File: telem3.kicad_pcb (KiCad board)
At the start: 4 copper layers, 124 x 80 mm, 200 parts, among them J1 STM32_TRACE, J10 Conn_01x04_Socket, J11 CAN_TERMINATION, J12 GPS_ANT, J3 EXPANSION_1, J4 ESP32_JTAG, J5 BAT, J6 STM_USBC, J7 Micro_SD_Card, J8 QT1, J9 QT2, Q1 2N7002, Q2 2N7002, Q3 2N7002, Q4 2N7002, Q5 2N7002, Q6 2N7002, Q7 IRLML9301, Q8 2N7002, SW1 RESET, SW2 OPT, SW3 ESP32_RST, SW4 GPS_RST, U1 STM32L562ZETx, U10 TCAN334G, U11 L80-R, U12 LSM6DS3, U13 BME280, U2 W25Q128JVS, U3 W25Q128JVS, U4 ESP32-C3-MINI-1, U5 TPS2116, U6 TPS54202DDC, U7 BQ24075RGT, U8 AP7361C-33E, U9 NUP4202, Y1 8MHz, Y2 32.768kHz

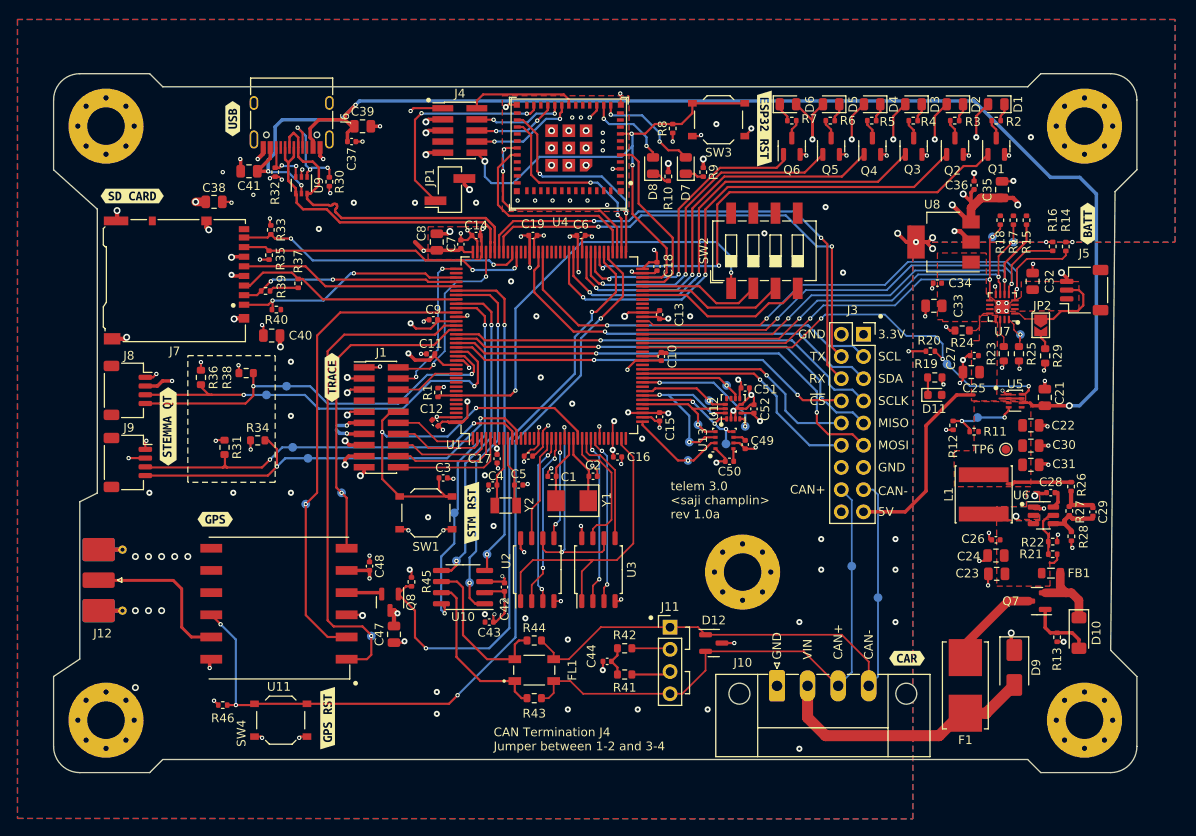
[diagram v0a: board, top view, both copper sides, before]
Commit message: fix uart gps
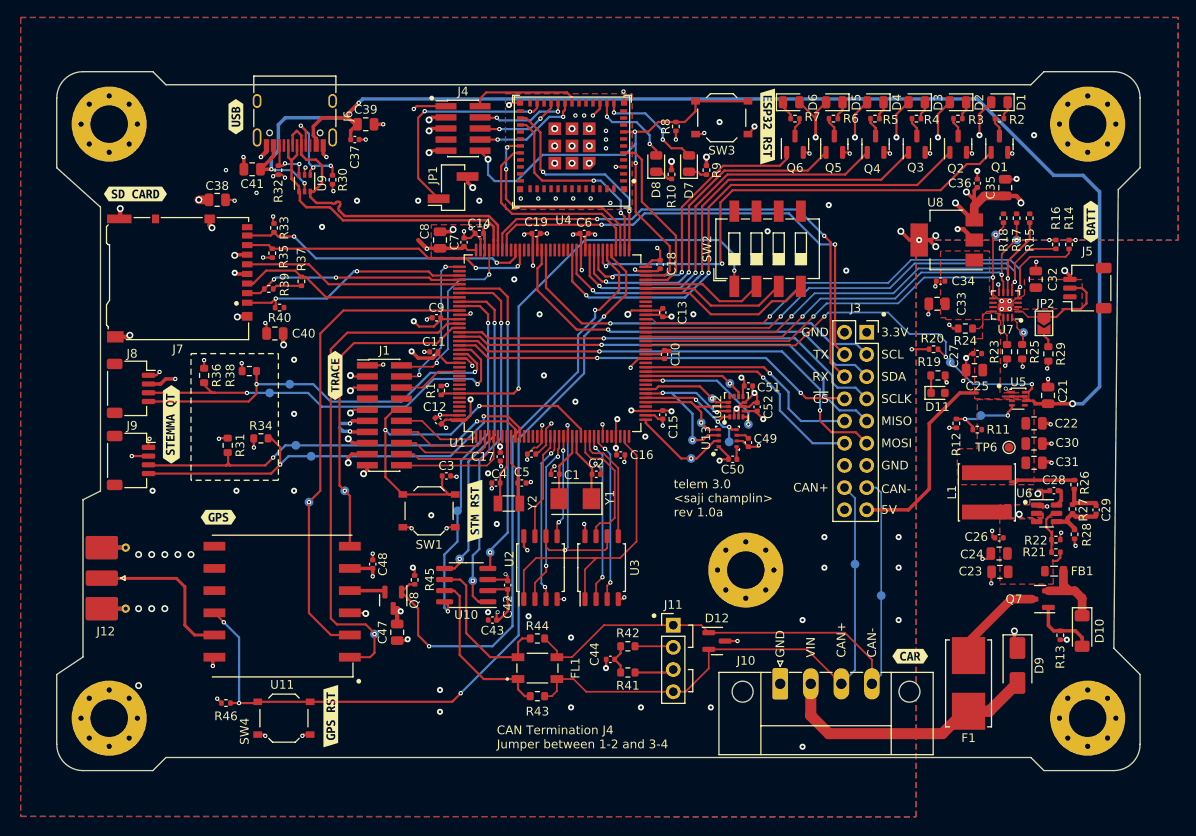
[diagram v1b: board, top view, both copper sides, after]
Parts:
- moved C1 0.43 mm to (139.1, 83.1)
- moved C11 0.43 mm to (125.2, 69.1)
- moved C12 0.43 mm to (125.7, 77.0)
- moved C13 0.43 mm to (151.4, 64.6)
- moved C15 0.43 mm to (151.4, 76.3)
- moved C2 0.43 mm to (143.8, 83.1)
- moved C20 0.43 mm to (136.3, 80.8)
- moved C22 0.43 mm to (193.9, 77.3)
- moved C24 0.43 mm to (189.9, 92.2)
- moved C28 0.43 mm to (196.1, 85.0)
- moved C29 0.43 mm to (201.0, 87.2)
- moved C30 0.43 mm to (193.9, 79.6)
- moved C31 0.43 mm to (193.9, 81.8)
- moved C4 0.43 mm to (132.3, 84.1)
- moved C40 0.43 mm to (107.0, 67.0)
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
